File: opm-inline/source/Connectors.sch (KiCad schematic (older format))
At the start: 34 parts, among them J1 Info, J2 VCC_IO, J3 PWMx6, J4 Fan, J6 Current Sensing, Q7 WSD90P06DN56, U2 TerminalBlock_2_P5.08mm, U3 TerminalBlock_3_P5.08mm

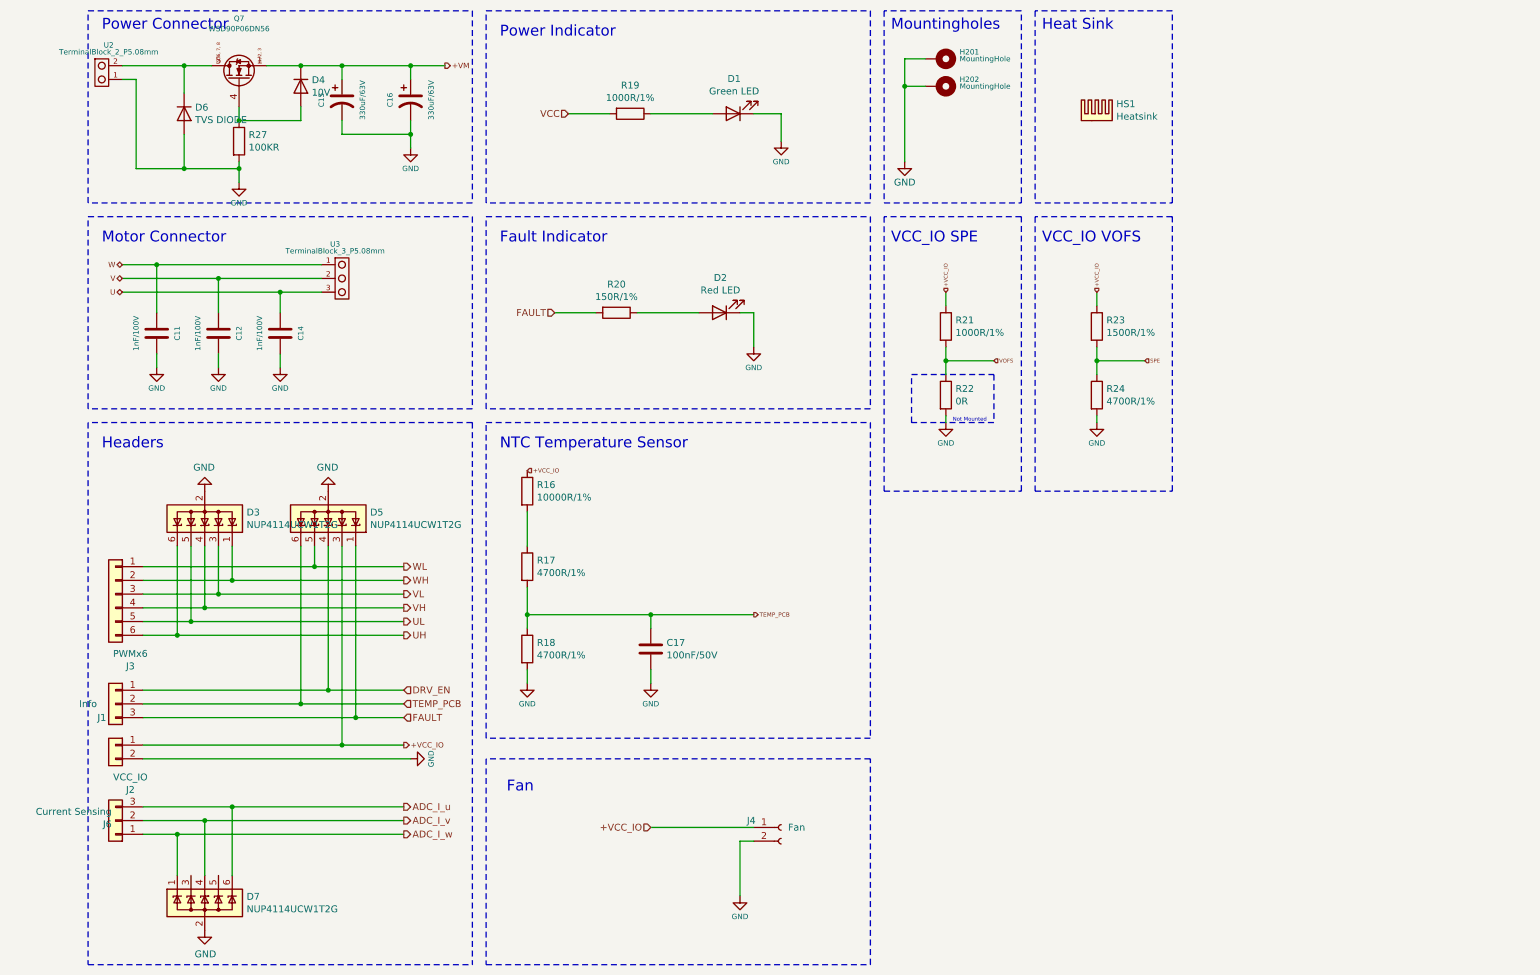
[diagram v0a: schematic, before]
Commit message: update
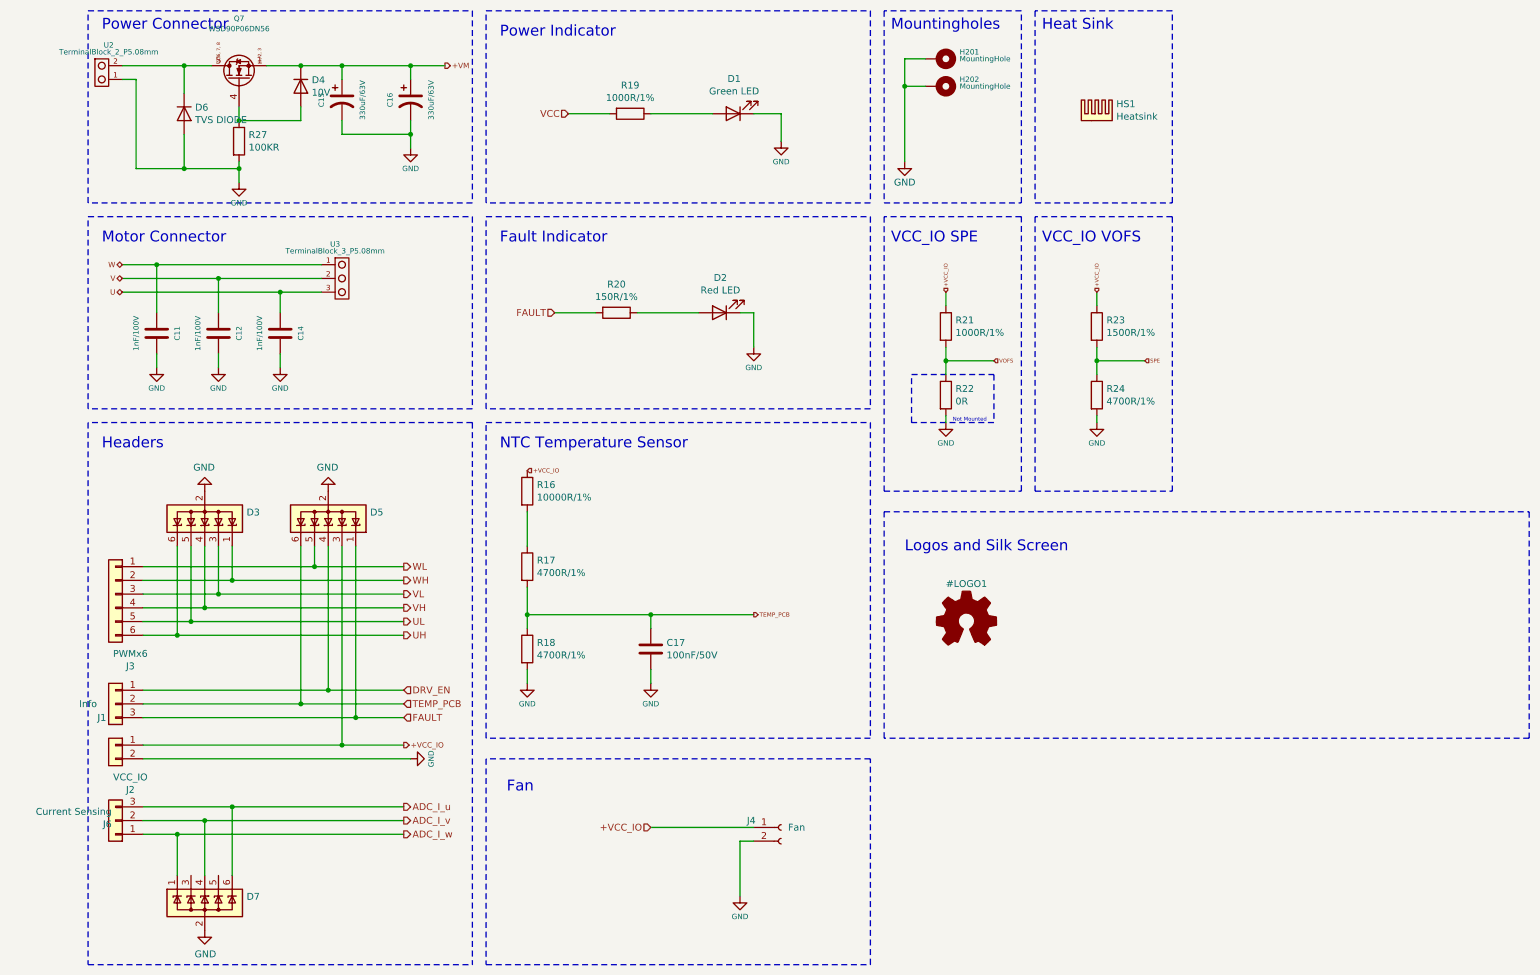
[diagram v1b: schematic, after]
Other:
- note added: "Logos and Silk Screen"
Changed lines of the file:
@@
 	7500 4250 8500 4250
-Wire Notes Line
-	8500 4250 8500 2250
 Wire Notes Line
 	8500 2250 7500 2250
@@
 P 2350 4450
 F 0 "D5" H 2045 4404 50  0000 R CNN
-F 1 "NUP4114UCW1T2G" H 2045 4495 50  0000 R CNN
+F 1 "NUP4114UCW1T2G" H 2045 4495 50  0001 R CNN
 F 2 "Libraries:NUP4114UCW1T2G" H 2650 4400 50  0001 L CNN
 F 3 "https://datasheet.lcsc.com/lcsc/2001031717_onsemi-NUP4114UCW1T2G_C463643.pdf" H 2475 4575 50  0001 C CNN
@@
 P 1450 4450
 F 0 "D3" H 1145 4404 50  0000 R CNN
-F 1 "NUP4114UCW1T2G" H 1145 4495 50  0000 R CNN
+F 1 "NUP4114UCW1T2G" H 1145 4495 50  0001 R CNN
 F 2 "Libraries:NUP4114UCW1T2G" H 1750 4400 50  0001 L CNN
 F 3 "https://datasheet.lcsc.com/lcsc/2001031717_onsemi-NUP4114UCW1T2G_C463643.pdf" H 1575 4575 50  0001 C CNN
@@
 P 1450 7250
 F 0 "D7" H 1755 7296 50  0000 L CNN
-F 1 "NUP4114UCW1T2G" H 1755 7205 50  0000 L CNN
+F 1 "NUP4114UCW1T2G" H 1755 7205 50  0001 L CNN
 F 2 "Libraries:NUP4114UCW1T2G" H 1750 7200 50  0001 L CNN
 F 3 "https://datasheet.lcsc.com/lcsc/2001031717_onsemi-NUP4114UCW1T2G_C463643.pdf" H 1575 7375 50  0001 C CNN
@@
 Wire Wire Line
 	2250 4800 2900 4800
+Wire Notes Line
+	11100 4400 11100 6050
+Wire Notes Line
+	11100 6050 6400 6050
+Wire Notes Line
+	6400 6050 6400 4400
+Wire Notes Line
+	6400 4400 11100 4400
+Wire Notes Line
+	8500 2250 8500 4250
+$Comp
+L Graphic:Logo_Open_Hardware_Small #LOGO1
+U 1 1 61E56420
+P 7000 5200
+F 0 "#LOGO1" H 7000 5475 50  0000 C CNN
+F 1 "Logo_Open_Hardware_Small" H 7000 4975 50  0001 C CNN
+F 2 "Symbol:OSHW-Logo2_9.8x8mm_SilkScreen" H 7000 5200 50  0001 C CNN
+F 3 "~" H 7000 5200 50  0001 C CNN
+	1    7000 5200
+	1    0    0    -1
+$EndComp
+Text Notes 6550 4700 0    79   ~ 0
+Logos and Silk Screen
 $EndSCHEMATC
